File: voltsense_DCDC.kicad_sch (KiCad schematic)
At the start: 9 parts, among them J18 Capacitor connector, U5 Opamp_Quad

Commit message: SCH Save: 4 files changed currsense_DCDC.kicad_sch 0/0/4 decoration.kicad_sch 0/0/12 voltsense_DCDC.kicad_sch 0/0/4 voltsense_inverter.kicad_sch 0/0/4
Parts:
- R33, R34, R35, R36: footprint Resistor_THT:R_Axial_DIN0207_L6.3mm_D2.5mm_P7.62mm_Horizontal -> (none)
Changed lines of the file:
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@@
 			)
 		)
-		(property "Footprint" "Resistor_THT:R_Axial_DIN0207_L6.3mm_D2.5mm_P7.62mm_Horizontal"
+		(property "Footprint" ""
 			(at 45.212 68.58 90)
 			(hide yes)
@@
 			)
 		)
-		(property "Footprint" "Resistor_THT:R_Axial_DIN0207_L6.3mm_D2.5mm_P7.62mm_Horizontal"
+		(property "Footprint" ""
 			(at 63.5 62.738 90)
 			(hide yes)
@@
 			)
 		)
-		(property "Footprint" "Resistor_THT:R_Axial_DIN0207_L6.3mm_D2.5mm_P7.62mm_Horizontal"
+		(property "Footprint" ""
 			(at 104.14 65.278 90)
 			(hide yes)
@@
 			)
 		)
-		(property "Footprint" "Resistor_THT:R_Axial_DIN0207_L6.3mm_D2.5mm_P7.62mm_Horizontal"
+		(property "Footprint" ""
 			(at 45.212 52.07 90)
 			(hide yes)

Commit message: SCH Save: 1 files changed voltsense_DCDC.kicad_sch 0/0/4
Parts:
- R33, R34, R35, R36: footprint (none) -> Resistor_THT:R_Axial_DIN0207_L6.3mm_D2.5mm_P7.62mm_Horizontal
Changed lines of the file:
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@@
 			)
 		)
-		(property "Footprint" ""
+		(property "Footprint" "Resistor_THT:R_Axial_DIN0207_L6.3mm_D2.5mm_P7.62mm_Horizontal"
 			(at 45.212 68.58 90)
 			(hide yes)
@@
 			)
 		)
-		(property "Footprint" ""
+		(property "Footprint" "Resistor_THT:R_Axial_DIN0207_L6.3mm_D2.5mm_P7.62mm_Horizontal"
 			(at 63.5 62.738 90)
 			(hide yes)
@@
 			)
 		)
-		(property "Footprint" ""
+		(property "Footprint" "Resistor_THT:R_Axial_DIN0207_L6.3mm_D2.5mm_P7.62mm_Horizontal"
 			(at 104.14 65.278 90)
 			(hide yes)
@@
 			)
 		)
-		(property "Footprint" ""
+		(property "Footprint" "Resistor_THT:R_Axial_DIN0207_L6.3mm_D2.5mm_P7.62mm_Horizontal"
 			(at 45.212 52.07 90)
 			(hide yes)

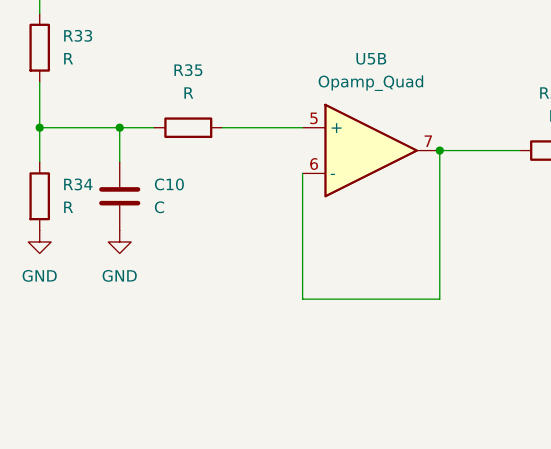
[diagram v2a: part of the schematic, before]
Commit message: Autosave
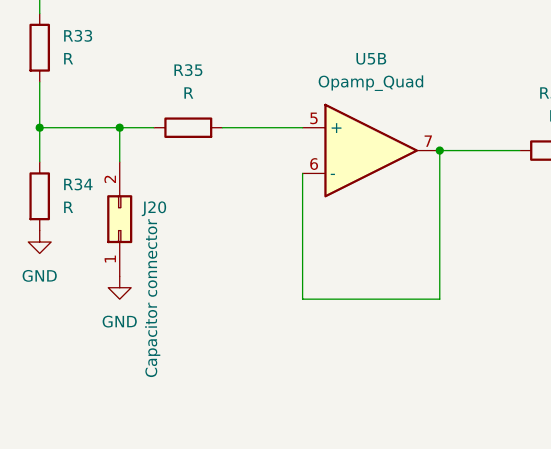
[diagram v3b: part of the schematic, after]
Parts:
- removed C10: C, symbol Device:C
- added J20: Capacitor connector, symbol Connector_Generic:Conn_02x01
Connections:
- net GND: now also J20.1 (Pin_1)
- net at R33.2, R34.1, R35.1: now also J20.2 (Pin_2)
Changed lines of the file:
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@@
-	)
-	(symbol
-		(lib_id "Device:C")
-		(at 55.88 68.58 0)
-		(unit 1)
-		(body_style 1)
-		(exclude_from_sim no)
-		(in_bom yes)
-		(on_board yes)
-		(in_pos_files yes)
-		(dnp no)
-		(fields_autoplaced yes)
-		(property "Reference" "C10"
-			(at 59.69 67.3099 0)
-			(show_name no)
-			(do_not_autoplace no)
-			(effects
-				(font
-					(size 1.27 1.27)
-				)
-				(justify left)
-			)
-		)
-		(property "Value" "C"
-			(at 59.69 69.8499 0)
-			(show_name no)
-			(do_not_autoplace no)
-			(effects
-				(font
-					(size 1.27 1.27)
-				)
-				(justify left)
-			)
-		)
-		(property "Footprint" ""
-			(at 56.8452 72.39 0)
-			(hide yes)
-			(show_name no)
-			(do_not_autoplace no)
-			(effects
-				(font
-					(size 1.27 1.27)
-				)
-			)
-		)
-		(property "Datasheet" ""
-			(at 55.88 68.58 0)
-			(hide yes)
-			(show_name no)
-			(do_not_autoplace no)
-			(effects
-				(font
-					(size 1.27 1.27)
-				)
-			)
-		)
-		(property "Description" "Unpolarized capacitor"
-			(at 55.88 68.58 0)
-			(hide yes)
-			(show_name no)
-			(do_not_autoplace no)
-			(effects
-				(font
-					(size 1.27 1.27)
-				)
-			)
-		)
-		(pin "1"
-		)
-		(pin "2"
-		)
-		(instances
-			(project "WET_PCB_v2"
-				(path "/13451c35-1666-47d9-9525-8d8125ba1cf3/a17383a4-d27f-4c25-9e0c-b0df1856b8d8"
-					(reference "C10")
-					(unit 1)
-				)
-			)
-		)
 	)
 	(symbol
 		(lib_id "power:GND")
-		(at 55.88 72.39 0)
+		(at 55.88 77.47 0)
 		(unit 1)
 		(body_style 1)
@@
 		(fields_autoplaced yes)
 		(property "Reference" "#PWR054"
-			(at 55.88 78.74 0)
+			(at 55.88 83.82 0)
 			(hide yes)
 			(show_name no)
@@
 		)
 		(property "Value" "GND"
+			(at 55.88 82.55 0)
+			(show_name no)
+			(do_not_autoplace no)
+			(effects
+				(font
+					(size 1.27 1.27)
+				)
+			)
+		)
+		(property "Footprint" ""
 			(at 55.88 77.47 0)
-			(show_name no)
-			(do_not_autoplace no)
-			(effects
-				(font
-					(size 1.27 1.27)
-				)
-			)
-		)
-		(property "Footprint" ""
-			(at 55.88 72.39 0)
 			(hide yes)
 			(show_name no)
@@
 		)
 		(property "Datasheet" ""
-			(at 55.88 72.39 0)
+			(at 55.88 77.47 0)
 			(hide yes)
 			(show_name no)
@@
 		)
 		(property "Description" "Power symbol creates a global label with name \"GND\" , ground"
-			(at 55.88 72.39 0)
+			(at 55.88 77.47 0)
 			(hide yes)
 			(show_name no)
@@
 					(unit 1)
 				)
+			)
+		)
+	)
+	(symbol
+		(lib_id "Connector_Generic:Conn_02x01")
+		(at 55.88 72.39 90)
+		(unit 1)
+		(body_style 1)
+		(exclude_from_sim no)
+		(in_bom yes)
+		(on_board yes)
+		(in_pos_files yes)
+		(dnp no)
+		(property "Reference" "J20"
+			(at 58.42 69.8499 90)
+			(show_name no)
+			(do_not_autoplace no)
+			(effects
+				(font
+					(size 1.27 1.27)
+				)
+				(justify right)
+			)
+		)
+		(property "Value" "Capacitor connector"
+			(at 59.436 71.12 0)
+			(show_name no)
+			(do_not_autoplace no)
+			(effects
+				(font
+					(size 1.27 1.27)
+				)
+				(justify right)
+			)
+		)
+		(property "Footprint" ""
+			(at 55.88 72.39 0)
+			(hide yes)
+			(show_name no)
+			(do_not_autoplace no)
+			(effects
+				(font
+					(size 1.27 1.27)
+				)
+			)
+		)
+		(property "Datasheet" ""
+			(at 55.88 72.39 0)
+			(hide yes)
+			(show_name no)
+			(do_not_autoplace no)
+			(effects
+				(font
+					(size 1.27 1.27)
+				)
+			)
+		)
+		(property "Description" "Generic connector, double row, 02x01, this symbol is compatible with counter-clockwise, top-bottom and odd-even numbering schemes., script generated (kicad-library-utils/schlib/autogen/connector/)"
+			(at 55.88 72.39 0)
+			(hide yes)
+			(show_name no)
+			(do_not_autoplace no)
+			(effects
+				(font
+					(size 1.27 1.27)
+				)
+			)
+		)
+		(pin "2"
+		)
+		(pin "1"
+		)
+		(instances
+			(project "WET_PCB_v2"
+				(path "/13451c35-1666-47d9-9525-8d8125ba1cf3/a17383a4-d27f-4c25-9e0c-b0df1856b8d8"
+					(reference "J20")
+					(unit 1)
+				)

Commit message: SCH Save: 3 files changed voltsense_DCDC.kicad_sch 156/0/87 voltsense_inverter.kicad_sch 0/0/2 WET_PCB_v2.kicad_pro 0/0/1
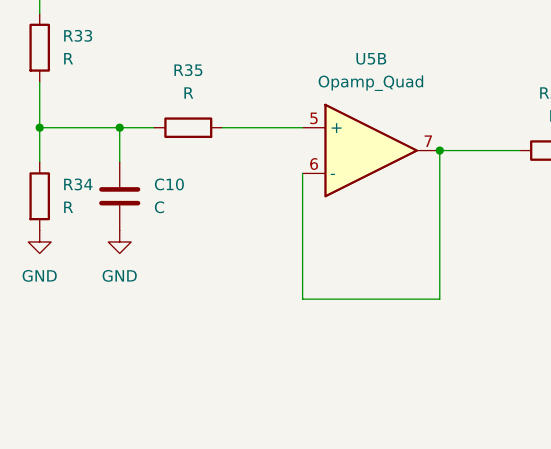
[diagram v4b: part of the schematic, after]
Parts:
- removed J20: Capacitor connector, symbol Connector_Generic:Conn_02x01
- added C10: C, symbol Device:C
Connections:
- net GND: now also C10.2
- net at R33.2, R34.1, R35.1: now also C10.1
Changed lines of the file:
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@@
+	)
+	(symbol
+		(lib_id "Device:C")
+		(at 55.88 68.58 0)
+		(unit 1)
+		(body_style 1)
+		(exclude_from_sim no)
+		(in_bom yes)
+		(on_board yes)
+		(in_pos_files yes)
+		(dnp no)
+		(fields_autoplaced yes)
+		(property "Reference" "C10"
+			(at 59.69 67.3099 0)
+			(show_name no)
+			(do_not_autoplace no)
+			(effects
+				(font
+					(size 1.27 1.27)
+				)
+				(justify left)
+			)
+		)
+		(property "Value" "C"
+			(at 59.69 69.8499 0)
+			(show_name no)
+			(do_not_autoplace no)
+			(effects
+				(font
+					(size 1.27 1.27)
+				)
+				(justify left)
+			)
+		)
+		(property "Footprint" ""
+			(at 56.8452 72.39 0)
+			(hide yes)
+			(show_name no)
+			(do_not_autoplace no)
+			(effects
+				(font
+					(size 1.27 1.27)
+				)
+			)
+		)
+		(property "Datasheet" ""
+			(at 55.88 68.58 0)
+			(hide yes)
+			(show_name no)
+			(do_not_autoplace no)
+			(effects
+				(font
+					(size 1.27 1.27)
+				)
+			)
+		)
+		(property "Description" "Unpolarized capacitor"
+			(at 55.88 68.58 0)
+			(hide yes)
+			(show_name no)
+			(do_not_autoplace no)
+			(effects
+				(font
+					(size 1.27 1.27)
+				)
+			)
+		)
+		(pin "1"
+		)
+		(pin "2"
+		)
+		(instances
+			(project "WET_PCB_v2"
+				(path "/13451c35-1666-47d9-9525-8d8125ba1cf3/a17383a4-d27f-4c25-9e0c-b0df1856b8d8"
+					(reference "C10")
+					(unit 1)
+				)
+			)
+		)
 	)
 	(symbol
 		(lib_id "power:GND")
-		(at 55.88 77.47 0)
+		(at 55.88 72.39 0)
 		(unit 1)
 		(body_style 1)
@@
 		(fields_autoplaced yes)
 		(property "Reference" "#PWR054"
-			(at 55.88 83.82 0)
+			(at 55.88 78.74 0)
 			(hide yes)
 			(show_name no)
@@
 		)
 		(property "Value" "GND"
-			(at 55.88 82.55 0)
+			(at 55.88 77.47 0)
 			(show_name no)
 			(do_not_autoplace no)
@@
 		)
 		(property "Footprint" ""
-			(at 55.88 77.47 0)
+			(at 55.88 72.39 0)
 			(hide yes)
 			(show_name no)
@@
 		)
 		(property "Datasheet" ""
-			(at 55.88 77.47 0)
+			(at 55.88 72.39 0)
 			(hide yes)
 			(show_name no)
@@
 		)
 		(property "Description" "Power symbol creates a global label with name \"GND\" , ground"
-			(at 55.88 77.47 0)
+			(at 55.88 72.39 0)
 			(hide yes)
 			(show_name no)
@@
 					(unit 1)
 				)
-			)
-		)
-	)
-	(symbol
-		(lib_id "Connector_Generic:Conn_02x01")
-		(at 55.88 72.39 90)
-		(unit 1)
-		(body_style 1)
-		(exclude_from_sim no)
-		(in_bom yes)
-		(on_board yes)
-		(in_pos_files yes)
-		(dnp no)
-		(property "Reference" "J20"
-			(at 58.42 69.8499 90)
-			(show_name no)
-			(do_not_autoplace no)
-			(effects
-				(font
-					(size 1.27 1.27)
-				)
-				(justify right)
-			)
-		)
-		(property "Value" "Capacitor connector"
-			(at 59.436 71.12 0)
-			(show_name no)
-			(do_not_autoplace no)
-			(effects
-				(font
-					(size 1.27 1.27)
-				)
-				(justify right)
-			)
-		)
-		(property "Footprint" ""
-			(at 55.88 72.39 0)
-			(hide yes)
-			(show_name no)
-			(do_not_autoplace no)
-			(effects
-				(font
-					(size 1.27 1.27)
-				)
-			)
-		)
-		(property "Datasheet" ""
-			(at 55.88 72.39 0)
-			(hide yes)
-			(show_name no)
-			(do_not_autoplace no)
-			(effects
-				(font
-					(size 1.27 1.27)
-				)
-			)
-		)
-		(property "Description" "Generic connector, double row, 02x01, this symbol is compatible with counter-clockwise, top-bottom and odd-even numbering schemes., script generated (kicad-library-utils/schlib/autogen/connector/)"
-			(at 55.88 72.39 0)
-			(hide yes)
-			(show_name no)
-			(do_not_autoplace no)
-			(effects
-				(font
-					(size 1.27 1.27)
-				)
-			)
-		)
-		(pin "2"
-		)
-		(pin "1"
-		)
-		(instances
-			(project "WET_PCB_v2"
-				(path "/13451c35-1666-47d9-9525-8d8125ba1cf3/a17383a4-d27f-4c25-9e0c-b0df1856b8d8"
-					(reference "J20")
-					(unit 1)
-				)
